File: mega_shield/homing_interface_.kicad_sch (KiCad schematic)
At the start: 4 parts, among them J2 T4040014031-000, J3 T4040014031-000

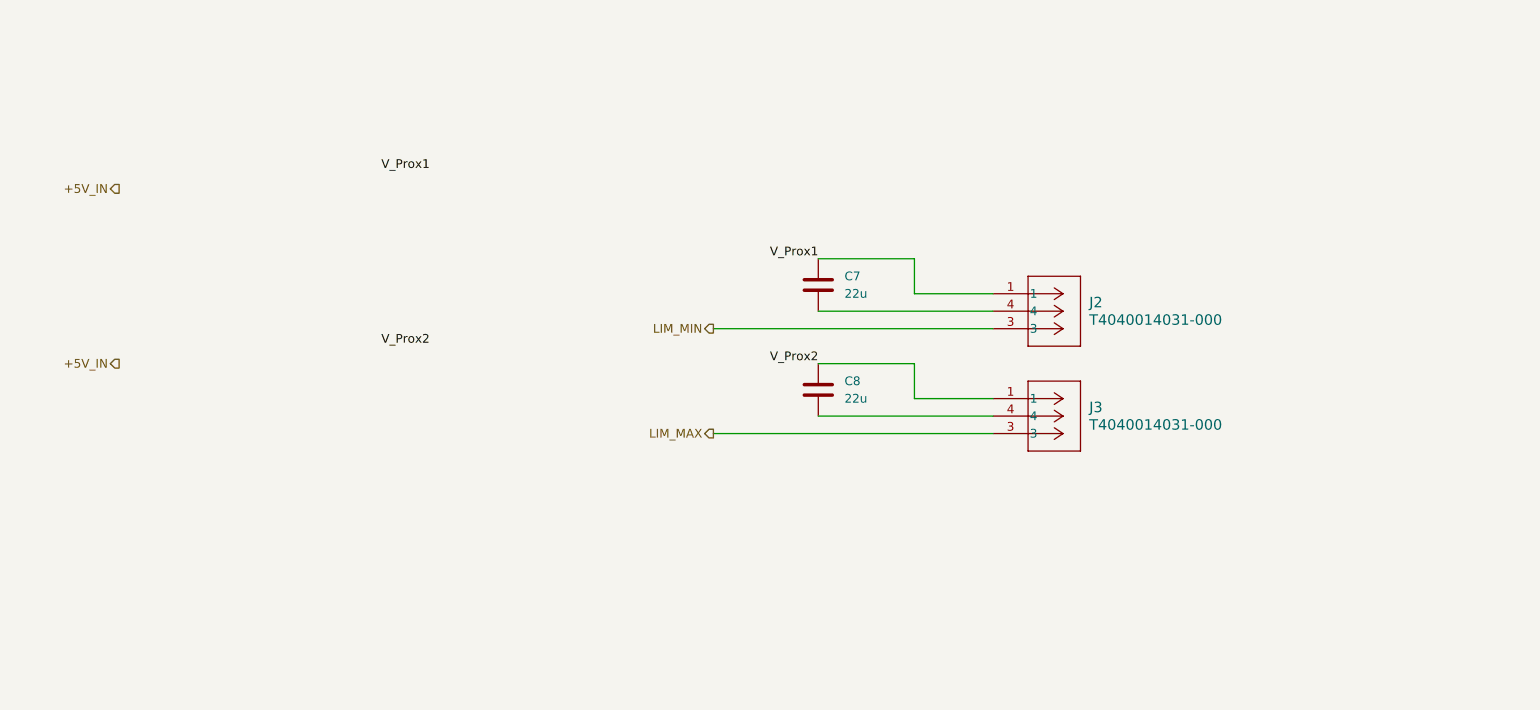
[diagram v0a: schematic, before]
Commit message: Adde note on sensor selection and reliability measures, adde homing interfaces for all servos.
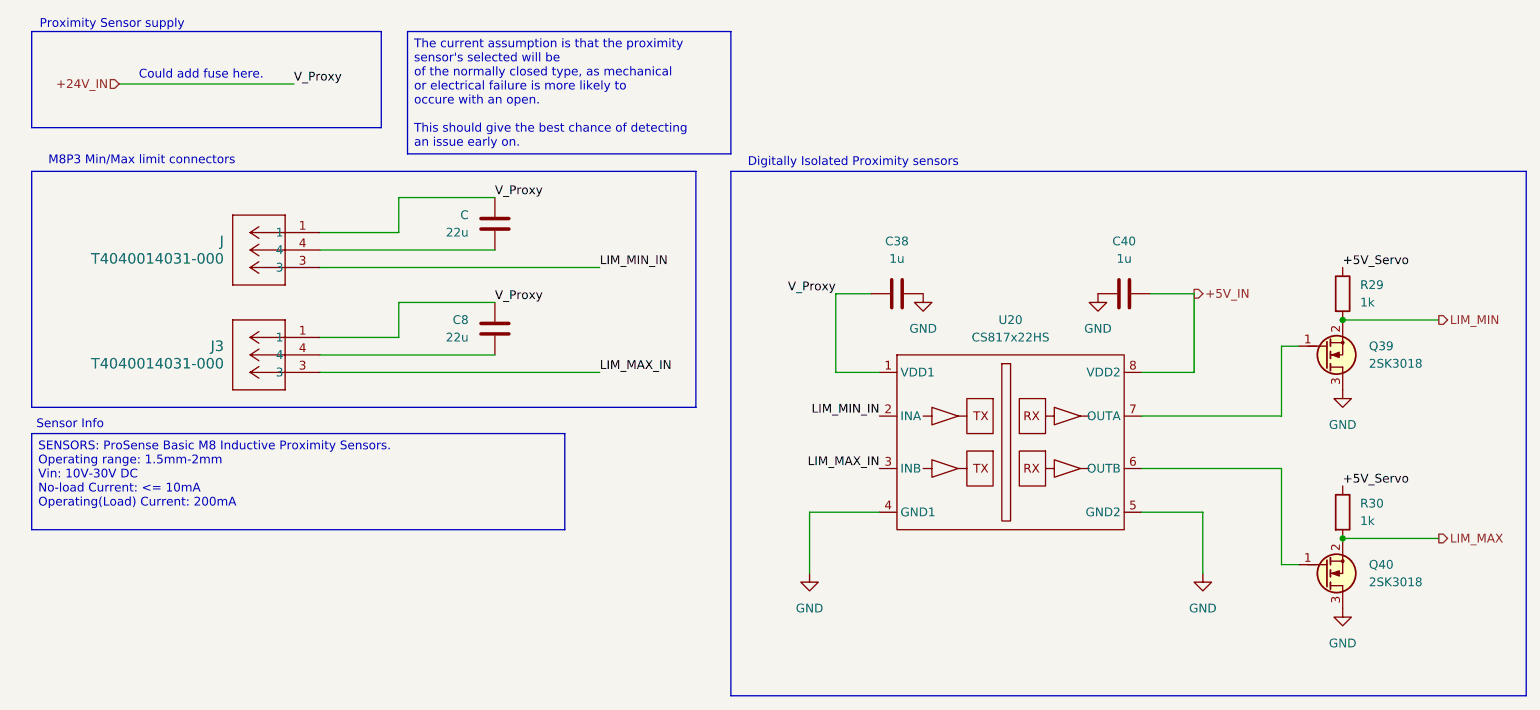
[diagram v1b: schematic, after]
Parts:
- added C38, C40: 1u, symbol Device:C
- added Q39, Q40: 2SK3018, PCM_Package_TO_SOT_SMD_AKL:SOT-323_SC-70, symbol PCM_Transistor_MOSFET_AKL:2SK3018
- added R29, R30: 1k, symbol Device:R
- added U20: CS817x22HS, Package_SO:SOIC-8_3.9x4.9mm_P1.27mm, symbol mega_shield:CS817x20HS
- renumbered C7 to C, J2 to J
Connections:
- net V_Prox2 is gone; now on net +24V_IN: C8.1, J3.1
- net +5V_IN: now also C40.2, U20.8 (VDD2)
- net LIM_MAX: now also Q40.2 (S), R30.2; no longer J3.3
- net LIM_MIN: now also Q39.2 (S), R29.2; no longer J.3
- net V_Prox1 renamed +24V_IN
- net +24V_IN: now also C38.1, U20.1 (VDD1)
- new net: Q39.1 (G), U20.7 (OUTA)
- new net: Q40.1 (G), U20.6 (OUTB)
- new net +5V_Servo: R29.1, R30.1
- new net GND: C38.2, C40.1, Q39.3 (D), Q40.3 (D), U20.4 (GND1), U20.5 (GND2)
- new net LIM_MAX_IN: J3.3, U20.3 (INB)
- new net LIM_MIN_IN: J.3, U20.2 (INA)
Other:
- note added: "Could add fuse here."
- note added: "Digitally Isolated Proximity sensors"
- note added: "M8P3 Min/Max limit connectors"
- note added: "Proximity Sensor supply"
- note added: "Sensor Info"
- moved on the sheet: C, C8, J, J3
